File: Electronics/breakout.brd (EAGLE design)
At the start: 28 x 69.2 mm, 7 parts, among them J1 FLATPACK2_CON, J4 FLATPACK2_DC_LUG, J5 FLATPACK2_DC_LUG, J6 FLATPACK2_DC_LUG, J7 FLATPACK2_DC_LUG

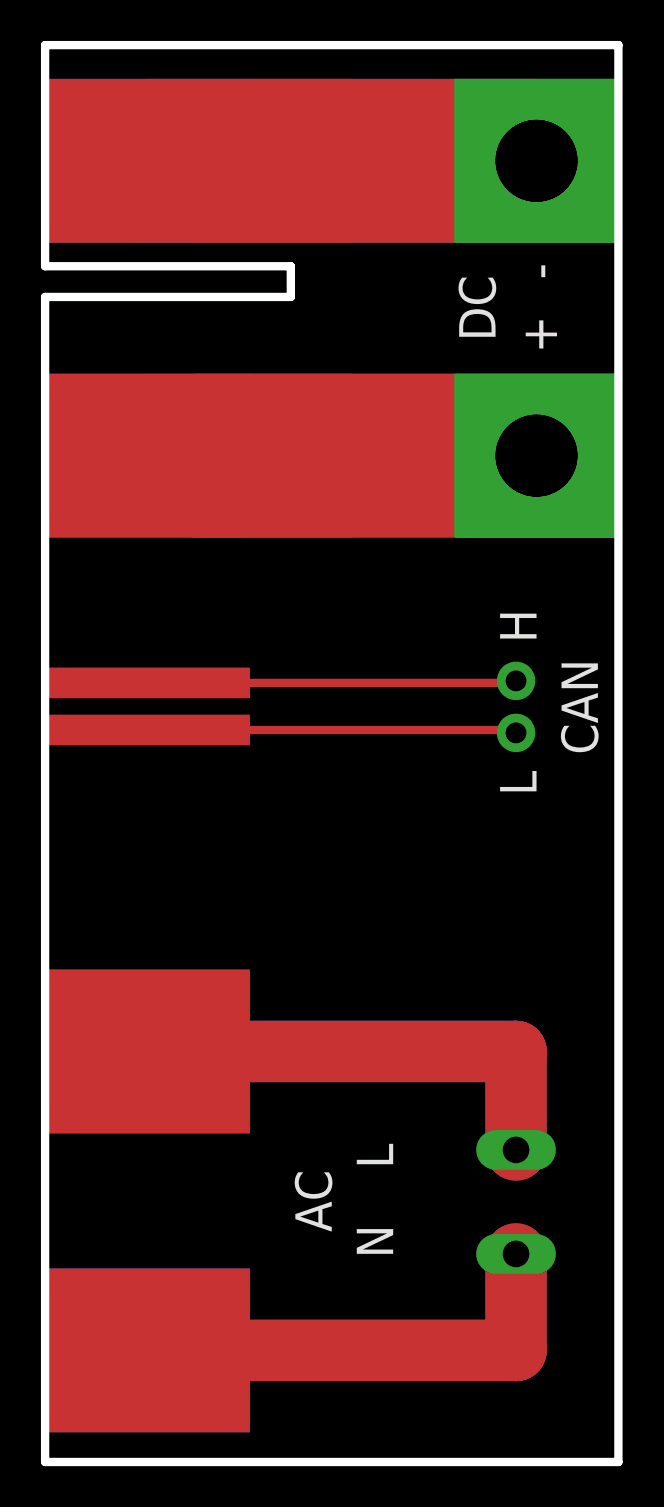
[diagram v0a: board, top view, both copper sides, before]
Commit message: Final revision of Flatpack breakout PCB
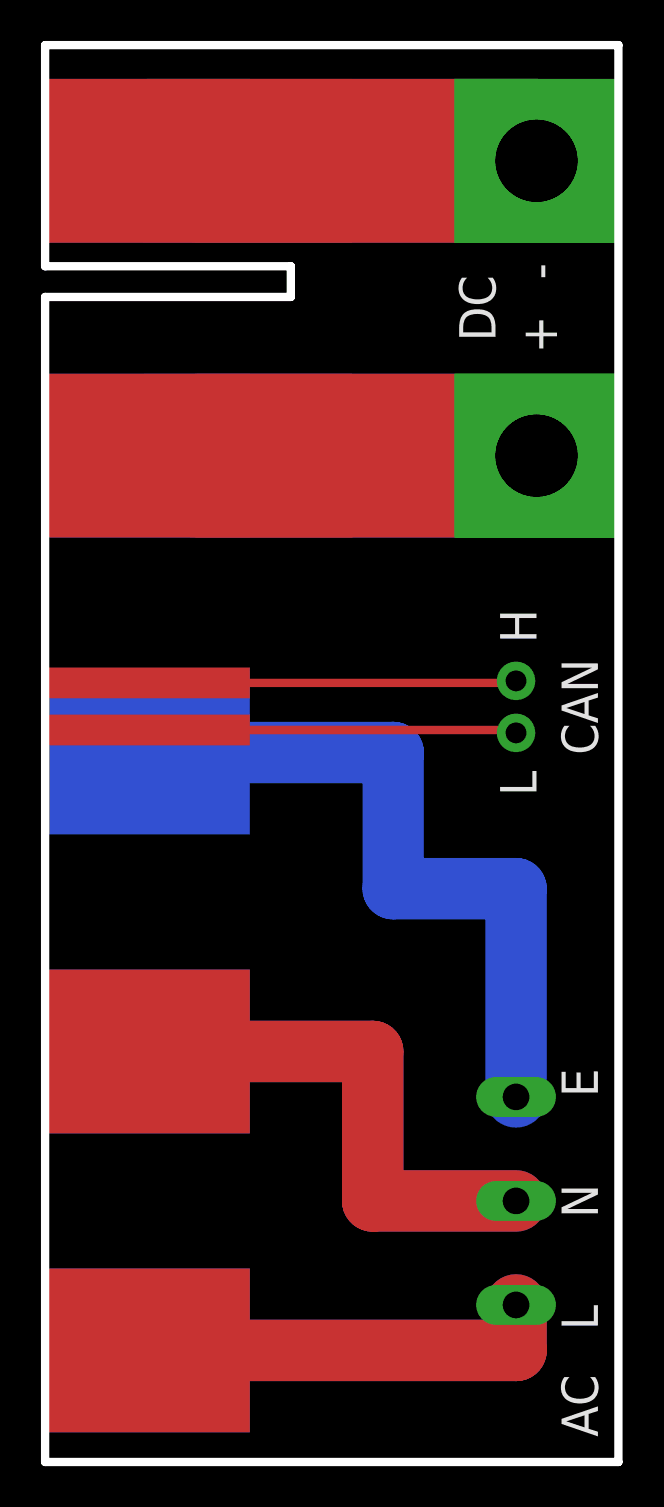
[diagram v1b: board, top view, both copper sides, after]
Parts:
- moved J2 0.05 mm to (23.0, 12.8)
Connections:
- new net N$6: J1.AC_EARTH, J2.3
- net N$3: now also J1.AC_LIVE_BOTTOM, J1.AC_LIVE_TOP, J2.1; no longer J1.AC_NEUTRAL_BOTTOM, J1.AC_NEUTRAL_TOP, J2.P2
- net N$4: now also J1.AC_NEUTRAL_BOTTOM, J1.AC_NEUTRAL_TOP, J2.2; no longer J1.AC_ACTIVE_BOTTOM, J1.AC_ACTIVE_TOP, J2.P1
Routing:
- net N$6: track 0.00 -> 34.8 mm
- net N$3: track 45.4 -> 40.4 mm
- net N$4: track 45.6 -> 50.6 mm
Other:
- board text added: "E"
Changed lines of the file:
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@@
 <layer number="21" name="tPlace" color="7" fill="1" visible="yes" active="yes"/>
 <layer number="22" name="bPlace" color="7" fill="1" visible="yes" active="yes"/>
-<layer number="23" name="tOrigins" color="15" fill="1" visible="no" active="yes"/>
-<layer number="24" name="bOrigins" color="15" fill="1" visible="no" active="yes"/>
+<layer number="23" name="tOrigins" color="15" fill="1" visible="yes" active="yes"/>
+<layer number="24" name="bOrigins" color="15" fill="1" visible="yes" active="yes"/>
 <layer number="25" name="tNames" color="7" fill="1" visible="yes" active="yes"/>
 <layer number="26" name="bNames" color="7" fill="1" visible="yes" active="yes"/>
 <layer number="27" name="tValues" color="7" fill="1" visible="yes" active="yes"/>
-<layer number="28" name="bValues" color="7" fill="1" visible="yes" active="yes"/>
+<layer number="28" name="bValues" color="7" fill="1" visible="no" active="yes"/>
 <layer number="29" name="tStop" color="7" fill="3" visible="no" active="yes"/>
 <layer number="30" name="bStop" color="7" fill="6" visible="no" active="yes"/>
@@
 <text x="25" y="58.55" size="1.778" layer="21" font="vector" rot="R90" align="bottom-right">-</text>
 <text x="22" y="56.35" size="1.778" layer="21" font="vector" rot="R90" align="bottom-center">DC</text>
-<text x="17" y="9.95" size="1.778" layer="21" font="vector" rot="R90">N</text>
-<text x="17" y="15.55" size="1.778" layer="21" font="vector" rot="R90" align="bottom-right">L</text>
-<text x="14" y="12.75" size="1.778" layer="21" font="vector" rot="R90" align="bottom-center">AC</text>
+<text x="27" y="12.75" size="1.778" layer="21" font="vector" rot="R90" align="bottom-center">N</text>
+<text x="27" y="7.67" size="1.778" layer="21" font="vector" rot="R90" align="bottom-right">L</text>
+<text x="27" y="2.75" size="1.778" layer="21" font="vector" rot="R90" align="bottom-center">AC</text>
+<text x="27" y="17.83" size="1.778" layer="21" font="vector" rot="R90">E</text>
 </plain>
 <attributes>
@@
 <attribute name="VALUE" x="21.222" y="39.42" size="0.6096" layer="27" font="vector" ratio="20" rot="R270"/>
 </element>
-<element name="J2" library="connectors" package="WEIDMULLER_PM_508" value="" x="23" y="12.7" rot="R180"/>
 <element name="J4" library="connectors" package="FLATPACK2_DC_LUG" value="FLATPACK2_DC_LUG" x="24" y="49.15" rot="MR0"/>
 <element name="J5" library="connectors" package="FLATPACK2_DC_LUG" value="FLATPACK2_DC_LUG" x="24" y="49.15"/>
 <element name="J6" library="connectors" package="FLATPACK2_DC_LUG" value="FLATPACK2_DC_LUG" x="24" y="63.55" rot="MR0"/>
 <element name="J7" library="connectors" package="FLATPACK2_DC_LUG" value="FLATPACK2_DC_LUG" x="24" y="63.55"/>
+<element name="J2" library="connectors" package="WEIDMULLER_PM_508" value="" x="23" y="12.75" rot="R180"/>
 </elements>
 <signals>
@@
 <wire x1="5" y1="35.75" x2="23" y2="35.75" width="0.4064" layer="1"/>
 <wire x1="23" y1="35.75" x2="23" y2="35.61" width="0.4064" layer="1"/>
-</signal>
-<signal name="N$3">
-<contactref element="J1" pad="AC_NEUTRAL_TOP"/>
-<contactref element="J1" pad="AC_NEUTRAL_BOTTOM"/>
-<contactref element="J2" pad="P2"/>
-<wire x1="5" y1="5.45" x2="23" y2="5.45" width="3" layer="1"/>
-<wire x1="23" y1="5.45" x2="23" y2="10.16" width="3" layer="1"/>
-<wire x1="5" y1="5.45" x2="23" y2="5.45" width="3" layer="16"/>
-<wire x1="23" y1="5.45" x2="23" y2="10.16" width="3" layer="16"/>
-</signal>
-<signal name="N$4">
-<contactref element="J2" pad="P1"/>
-<contactref element="J1" pad="AC_ACTIVE_BOTTOM"/>
-<contactref element="J1" pad="AC_ACTIVE_TOP"/>
-<wire x1="5" y1="20.05" x2="23" y2="20.05" width="3" layer="1"/>
-<wire x1="23" y1="20.05" x2="23" y2="15.24" width="3" layer="1"/>
-<wire x1="5" y1="20.05" x2="23" y2="20.05" width="3" layer="16"/>
-<wire x1="23" y1="20.05" x2="23" y2="15.24" width="3" layer="16"/>
 </signal>
 <signal name="N$5">
@@
 <wire x1="24" y1="63.55" x2="24" y2="63.55" width="0" layer="19" extent="1-16"/>
 </signal>
+<signal name="N$3">
+<contactref element="J1" pad="AC_LIVE_BOTTOM"/>
+<contactref element="J1" pad="AC_LIVE_TOP"/>
+<contactref element="J2" pad="1"/>
+<wire x1="5" y1="5.45" x2="23" y2="5.45" width="3" layer="1"/>
+<wire x1="23" y1="5.45" x2="23" y2="7.67" width="3" layer="1"/>
+<wire x1="5" y1="5.45" x2="23" y2="5.45" width="3" layer="16"/>
+<wire x1="23" y1="5.45" x2="23" y2="7.67" width="3" layer="16"/>
+</signal>
+<signal name="N$4">
+<contactref element="J2" pad="2"/>
+<contactref element="J1" pad="AC_NEUTRAL_BOTTOM"/>
+<contactref element="J1" pad="AC_NEUTRAL_TOP"/>
+<wire x1="5" y1="20.05" x2="16" y2="20.05" width="3" layer="1"/>
+<wire x1="16" y1="20.05" x2="16" y2="12.75" width="3" layer="1"/>
+<wire x1="16" y1="12.75" x2="23" y2="12.75" width="3" layer="1"/>
+<wire x1="5" y1="20.05" x2="16" y2="20.05" width="3" layer="16"/>
+<wire x1="16" y1="20.05" x2="16" y2="12.75" width="3" layer="16"/>
+<wire x1="16" y1="12.75" x2="23" y2="12.75" width="3" layer="16"/>
+</signal>
+<signal name="N$6">
+<contactref element="J1" pad="AC_EARTH"/>
+<contactref element="J2" pad="3"/>
+<wire x1="5" y1="34.65" x2="17" y2="34.65" width="3" layer="16"/>
+<wire x1="17" y1="34.65" x2="17" y2="28" width="3" layer="16"/>
+<wire x1="17" y1="28" x2="23" y2="28" width="3" layer="16"/>
+<wire x1="23" y1="28" x2="23" y2="17.83" width="3" layer="16"/>
+</signal>
 </signals>
+<errors>
+</errors>
 </board>
 </drawing>
